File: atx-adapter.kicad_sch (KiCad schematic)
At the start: 1 part

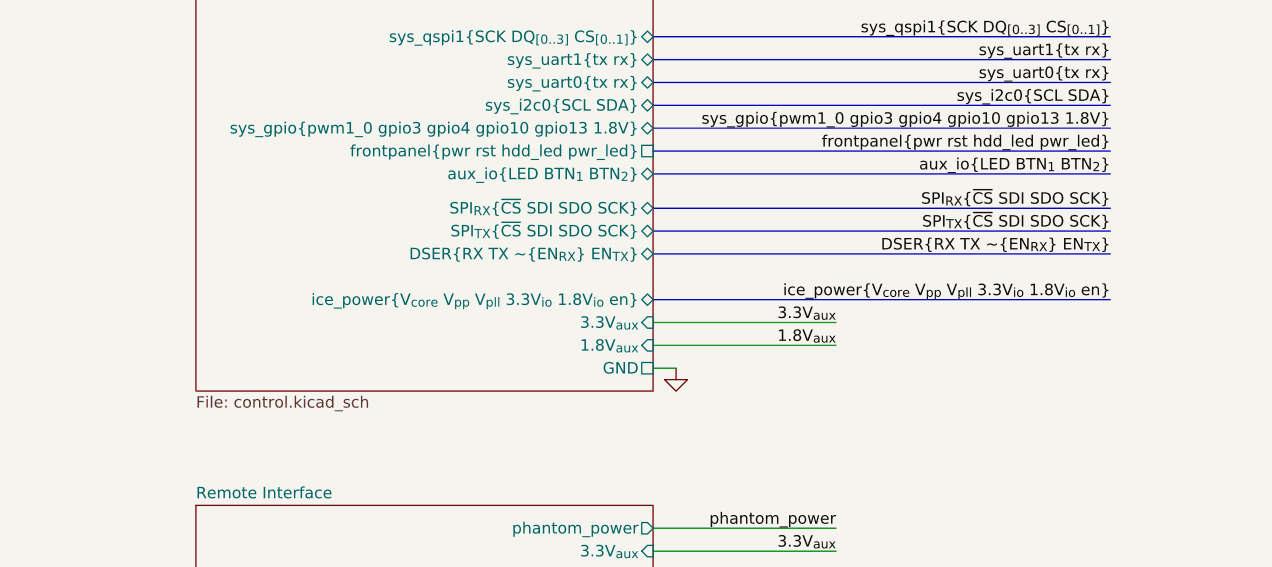
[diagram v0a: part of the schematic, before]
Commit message: tweak schematic
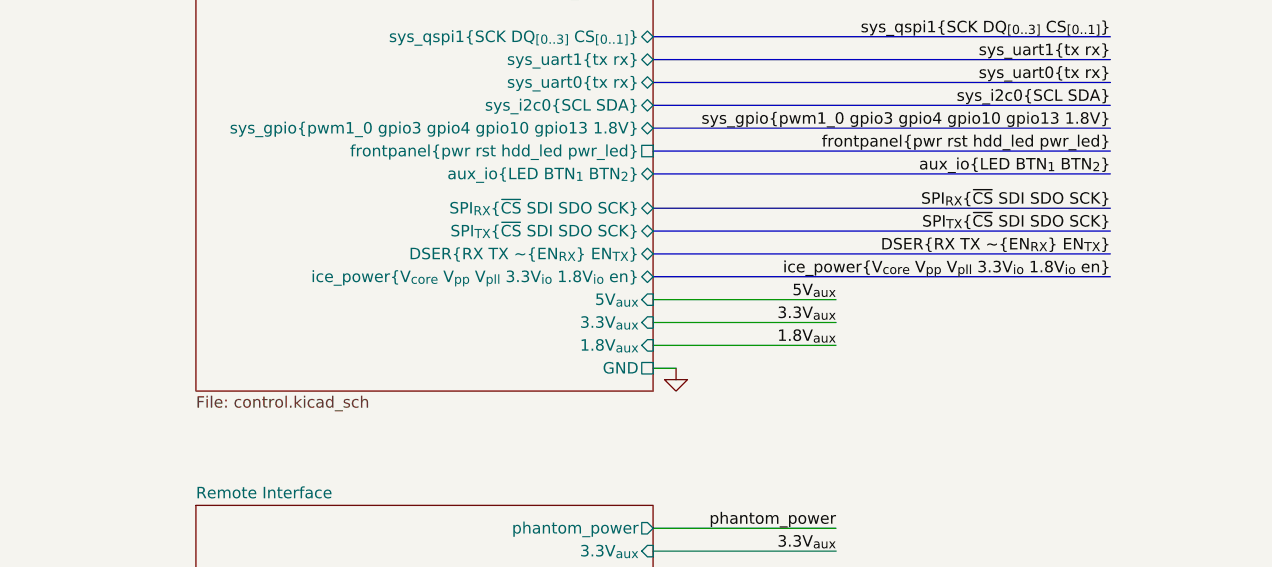
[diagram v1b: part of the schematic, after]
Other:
- sheet Control Logic ports: added 5V_{aux}; removed none
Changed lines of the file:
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@@
+    (stroke (width 0) (type solid) (color 0 0 0 0))
+  )
+  (wire (pts (xy 88.9 68.58) (xy 109.22 68.58))
     (stroke (width 0) (type solid) (color 0 0 0 0))
   )
@@
     (stroke (width 0) (type solid) (color 0 0 0 0))
   )
-  (bus (pts (xy 88.9 68.58) (xy 139.7 68.58))
+  (bus (pts (xy 88.9 66.04) (xy 139.7 66.04))
     (stroke (width 0) (type solid) (color 0 0 0 0))
   )
@@
   )
   (label "pgood_{main}" (at 109.22 22.86 180)
+    (effects (font (size 1.27 1.27)) (justify right bottom))
+  )
+  (label "5V_{aux}" (at 109.22 68.58 180)
     (effects (font (size 1.27 1.27)) (justify right bottom))
   )
@@
   )
   (label "ice_power{V_{core} V_{pp} V_{pll} 3.3V_{io} 1.8V_{io} en}"
-    (at 139.7 68.58 0)
+    (at 139.7 66.04 0)
     (effects (font (size 1.27 1.27)) (justify right bottom))
   )
@@
     (pin "1")
   )
-  (symbol (lib_name "proj_sym:GND_4") (lib_id "proj_sym:GND") (at 91.44 76.2 0) (unit 1)
+  (symbol (lib_id "proj_sym:GND") (at 91.44 76.2 0) (unit 1)
     (in_bom yes) (on_board yes) (fields_autoplaced)
     (property "Reference" "#PWR0101" (id 0) (at 91.44 82.55 0)
@@
     (pin "1")
   )
-  (symbol (lib_name "proj_sym:GND_3") (lib_id "proj_sym:GND") (at 91.44 114.3 0) (unit 1)
+  (symbol (lib_id "proj_sym:GND") (at 91.44 114.3 0) (unit 1)
     (in_bom yes) (on_board yes) (fields_autoplaced)
     (property "Reference" "#PWR0102" (id 0) (at 91.44 120.65 0)
@@
     (pin "1")
   )
-  (symbol (lib_name "proj_sym:GND_2") (lib_id "proj_sym:GND") (at 91.44 165.1 0) (unit 1)
+  (symbol (lib_id "proj_sym:GND") (at 91.44 165.1 0) (unit 1)
     (in_bom yes) (on_board yes) (fields_autoplaced)
     (property "Reference" "#PWR0104" (id 0) (at 91.44 171.45 0)
@@
     (pin "1")
   )
-  (symbol (lib_name "proj_sym:GND_1") (lib_id "proj_sym:GND") (at 161.29 142.24 0) (unit 1)
+  (symbol (lib_id "proj_sym:GND") (at 161.29 142.24 0) (unit 1)
     (in_bom yes) (on_board yes)
     (property "Reference" "#PWR0105" (id 0) (at 161.29 148.59 0)
@@
     (pin "1")
   )
-  (symbol (lib_name "proj_sym:GND_4") (lib_id "proj_sym:GND") (at 208.28 77.47 0) (unit 1)
+  (symbol (lib_id "proj_sym:GND") (at 208.28 77.47 0) (unit 1)
     (in_bom yes) (on_board yes) (fields_autoplaced)
     (property "Reference" "#PWR0107" (id 0) (at 208.28 83.82 0)
@@
     (pin "1")
   )
-  (symbol (lib_name "proj_sym:GND_2") (lib_id "proj_sym:GND") (at 208.28 166.37 0) (unit 1)
+  (symbol (lib_id "proj_sym:GND") (at 208.28 166.37 0) (unit 1)
     (in_bom yes) (on_board yes) (fields_autoplaced)
     (property "Reference" "#PWR0110" (id 0) (at 208.28 172.72 0)
@@
       (effects (font (size 1.27 1.27)) (justify right))
     )
-    (pin "ice_power{V_{core} V_{pp} V_{pll} 3.3V_{io} 1.8V_{io} en}" bidirectional (at 88.9 68.58 0)
+    (pin "ice_power{V_{core} V_{pp} V_{pll} 3.3V_{io} 1.8V_{io} en}" bidirectional (at 88.9 66.04 0)
       (effects (font (size 1.27 1.27)) (justify right))
     )
@@
     )
     (pin "DSER{RX TX ~EN_{RX} EN_{TX}}" bidirectional (at 88.9 63.5 0)
+      (effects (font (size 1.27 1.27)) (justify right))
+    )
+    (pin "5V_{aux}" input (at 88.9 68.58 0)
       (effects (font (size 1.27 1.27)) (justify right))
     )
@@
     (path "/72ab637e-73d9-486d-888e-3c2c6270d9a8/bc72db2b-9f5f-4ba6-8232-ff8f0707c04e" (page "12"))
     (path "/72ab637e-73d9-486d-888e-3c2c6270d9a8/fe1a7ea6-291d-47c4-9489-cbe0d1c0cfae" (page "13"))
+    (path "/ca64c4b8-5526-412c-b79b-5b6fc95e3044/27932af1-860c-416d-962f-4fa931a00a4e" (page "14"))
   )
   (symbol_instances
@@
     )
     (path "/72ab637e-73d9-486d-888e-3c2c6270d9a8/9603f169-6440-4ef6-ac65-ff267341ad51"
-      (reference "Q501") (unit 1) (value "Si2374DS") (footprint "")
+      (reference "Q501") (unit 1) (value "FDV301N") (footprint "")
     )
     (path "/72ab637e-73d9-486d-888e-3c2c6270d9a8/56e0358a-1de4-4866-93f7-73ad2101a78c"
@@
       (reference "R101") (unit 1) (value "15k 5%") (footprint "")
     )
+    (path "/ca64c4b8-5526-412c-b79b-5b6fc95e3044/8a622ab9-e00a-44fe-8fc6-b49fda12ae18"
+      (reference "R201") (unit 1) (value "41k2") (footprint "")
+    )
+    (path "/ca64c4b8-5526-412c-b79b-5b6fc95e3044/cd57e2d6-bb75-4703-940c-f2ff2fedc93b"
+      (reference "R202") (unit 1) (value "11k5") (footprint "")
+    )
+    (path "/ca64c4b8-5526-412c-b79b-5b6fc95e3044/6b13a45c-2e12-4db7-a179-d1354d3e1bdd"
+      (reference "R203") (unit 1) (value "20k") (footprint "")
+    )
+    (path "/ca64c4b8-5526-412c-b79b-5b6fc95e3044/c46195be-1b47-4e8d-bf50-2a45130f966f"
+      (reference "R204") (unit 1) (value "10k") (footprint "")
+    )
+    (path "/ca64c4b8-5526-412c-b79b-5b6fc95e3044/1619d19d-3e4e-4ec6-878d-cc9259c914aa"
+      (reference "R205") (unit 1) (value "20k") (footprint "")
+    )
+    (path "/ca64c4b8-5526-412c-b79b-5b6fc95e3044/6b233d81-c058-44a4-8940-38164c853674"
+      (reference "R206") (unit 1) (value "10k") (footprint "")
+    )
     (path "/d88ec964-55e1-4732-98a1-1ae5dd79106c/9607caeb-8126-41c9-b966-85bd399924ca"
       (reference "R301") (unit 1) (value "1k4") (footprint "")
@@
       (reference "R1201") (unit 1) (value "100k") (footprint "")
     )
-    (path "/ca64c4b8-5526-412c-b79b-5b6fc95e3044/6b13a45c-2e12-4db7-a179-d1354d3e1bdd"
-      (reference "R?") (unit 1) (value "20k") (footprint "")
-    )
-    (path "/ca64c4b8-5526-412c-b79b-5b6fc95e3044/8a622ab9-e00a-44fe-8fc6-b49fda12ae18"
-      (reference "R?") (unit 1) (value "41k2") (footprint "")
-    )
-    (path "/ca64c4b8-5526-412c-b79b-5b6fc95e3044/c46195be-1b47-4e8d-bf50-2a45130f966f"
-      (reference "R?") (unit 1) (value "10k") (footprint "")
-    )
-    (path "/ca64c4b8-5526-412c-b79b-5b6fc95e3044/cd57e2d6-bb75-4703-940c-f2ff2fedc93b"
-      (reference "R?") (unit 1) (value "11k5") (footprint "")
-    )
     (path "/ca64c4b8-5526-412c-b79b-5b6fc95e3044/9aca8fd9-1ab3-4cb4-9dfe-b6280a4d2849"
       (reference "RN201") (unit 1) (value "10k") (footprint "")
@@
       (reference "T301") (unit 4) (value "HX6062NL") (footprint "")
     )
-    (path "/ca64c4b8-5526-412c-b79b-5b6fc95e3044/7db0a8e8-3c69-4a64-a7ee-35179c7bae3a"
-      (reference "U201") (unit 1) (value "ICE40HX8K-BG121") (footprint "Package_BGA:BGA-121_9.0x9.0mm_Layout11x11_P0.8mm_Ball0.4mm_Pad0.35mm_NSMD")
-    )
-    (path "/ca64c4b8-5526-412c-b79b-5b6fc95e3044/c7b70689-4365-4151-a862-c4d8a442b3be"
-      (reference "U201") (unit 2) (value "ICE40HX8K-BG121") (footprint "Package_BGA:BGA-121_9.0x9.0mm_Layout11x11_P0.8mm_Ball0.4mm_Pad0.35mm_NSMD")
-    )
-    (path "/ca64c4b8-5526-412c-b79b-5b6fc95e3044/1e1b329e-7034-4951-a8b6-e5f0e76b552e"
-      (reference "U201") (unit 3) (value "ICE40HX8K-BG121") (footprint "Package_BGA:BGA-121_9.0x9.0mm_Layout11x11_P0.8mm_Ball0.4mm_Pad0.35mm_NSMD")
-    )
-    (path "/ca64c4b8-5526-412c-b79b-5b6fc95e3044/ead21deb-0eb3-4bec-9b87-cf057d30a19d"
-      (reference "U201") (unit 4) (value "ICE40HX8K-BG121") (footprint "Package_BGA:BGA-121_9.0x9.0mm_Layout11x11_P0.8mm_Ball0.4mm_Pad0.35mm_NSMD")
-    )
-    (path "/ca64c4b8-5526-412c-b79b-5b6fc95e3044/4922bc92-b92f-47a9-8454-6042c1580859"
-      (reference "U201") (unit 5) (value "ICE40HX8K-BG121") (footprint "Package_BGA:BGA-121_9.0x9.0mm_Layout11x11_P0.8mm_Ball0.4mm_Pad0.35mm_NSMD")
-    )
     (path "/ca64c4b8-5526-412c-b79b-5b6fc95e3044/ab1e45e0-2655-40cd-bcf8-94d4fabc4371"
-      (reference "U202") (unit 1) (value "TMUX1104") (footprint "")
+      (reference "U201") (unit 1) (value "TMUX1104") (footprint "")
     )
     (path "/ca64c4b8-5526-412c-b79b-5b6fc95e3044/78d25d96-6dac-4e26-a19a-bfffc4e089c2"
-      (reference "U203") (unit 1) (value "SLG46621") (footprint "")
+      (reference "U202") (unit 1) (value "SLG46621") (footprint "")
     )
     (path "/d88ec964-55e1-4732-98a1-1ae5dd79106c/866280ba-ce33-4925-b72c-4502bd6f46d4"
@@
       (reference "U1301") (unit 1) (value "MPM3811") (footprint "")
     )
-  )
+    (path "/ca64c4b8-5526-412c-b79b-5b6fc95e3044/27932af1-860c-416d-962f-4fa931a00a4e/a43dd9ef-0b03-4468-9454-771bc448fd28"
+      (reference "U1401") (unit 1) (value "ICE40HX8K-BG121") (footprint "Package_BGA:BGA-121_9.0x9.0mm_Layout11x11_P0.8mm_Ball0.4mm_Pad0.35mm_NSMD")
+    )
+    (path "/ca64c4b8-5526-412c-b79b-5b6fc95e3044/27932af1-860c-416d-962f-4fa931a00a4e/0d704281-6b81-4f86-85ab-3913ecdfdab4"
+      (reference "U1401") (unit 2) (value "ICE40HX8K-BG121") (footprint "Package_BGA:BGA-121_9.0x9.0mm_Layout11x11_P0.8mm_Ball0.4mm_Pad0.35mm_NSMD")
+    )
+    (path "/ca64c4b8-5526-412c-b79b-5b6fc95e3044/27932af1-860c-416d-962f-4fa931a00a4e/19427866-29d7-45c1-aa68-bb1dc22853fd"
+      (reference "U1401") (unit 3) (value "ICE40HX8K-BG121") (footprint "Package_BGA:BGA-121_9.0x9.0mm_Layout11x11_P0.8mm_Ball0.4mm_Pad0.35mm_NSMD")
+    )
+    (path "/ca64c4b8-5526-412c-b79b-5b6fc95e3044/27932af1-860c-416d-962f-4fa931a00a4e/8f5c0dda-9869-49a9-b84f-edb28b0063c3"
+      (reference "U1401") (unit 4) (value "ICE40HX8K-BG121") (footprint "Package_BGA:BGA-121_9.0x9.0mm_Layout11x11_P0.8mm_Ball0.4mm_Pad0.35mm_NSMD")
+    )
+    (path "/ca64c4b8-5526-412c-b79b-5b6fc95e3044/27932af1-860c-416d-962f-4fa931a00a4e/829fdc55-9676-4362-9443-16266628cfda"
+      (reference "U1401") (unit 5) (value "ICE40HX8K-BG121") (footprint "Package_BGA:BGA-121_9.0x9.0mm_Layout11x11_P0.8mm_Ball0.4mm_Pad0.35mm_NSMD")
+    )
+  )
